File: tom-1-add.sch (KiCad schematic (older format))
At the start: 5 parts, among them J9 Conn_02x08_Top_Bottom, U12 74LS283, U13 74LS283, U18 74LS283, U19 74LS283

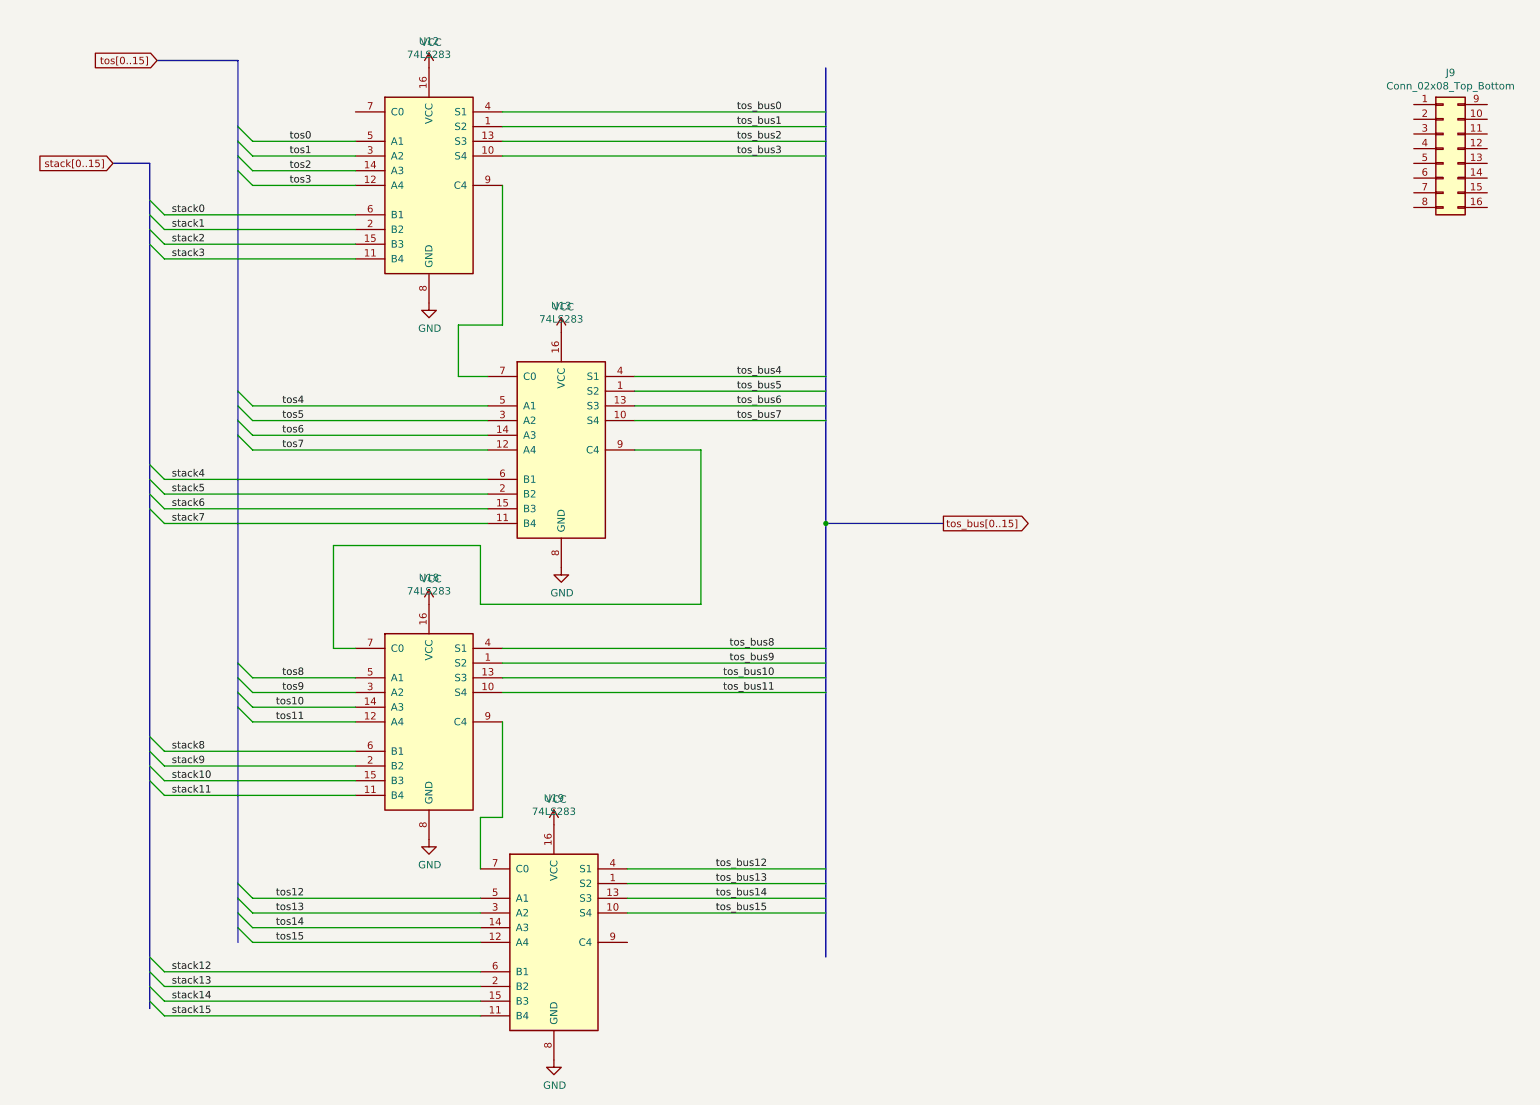
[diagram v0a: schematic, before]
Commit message: Next level
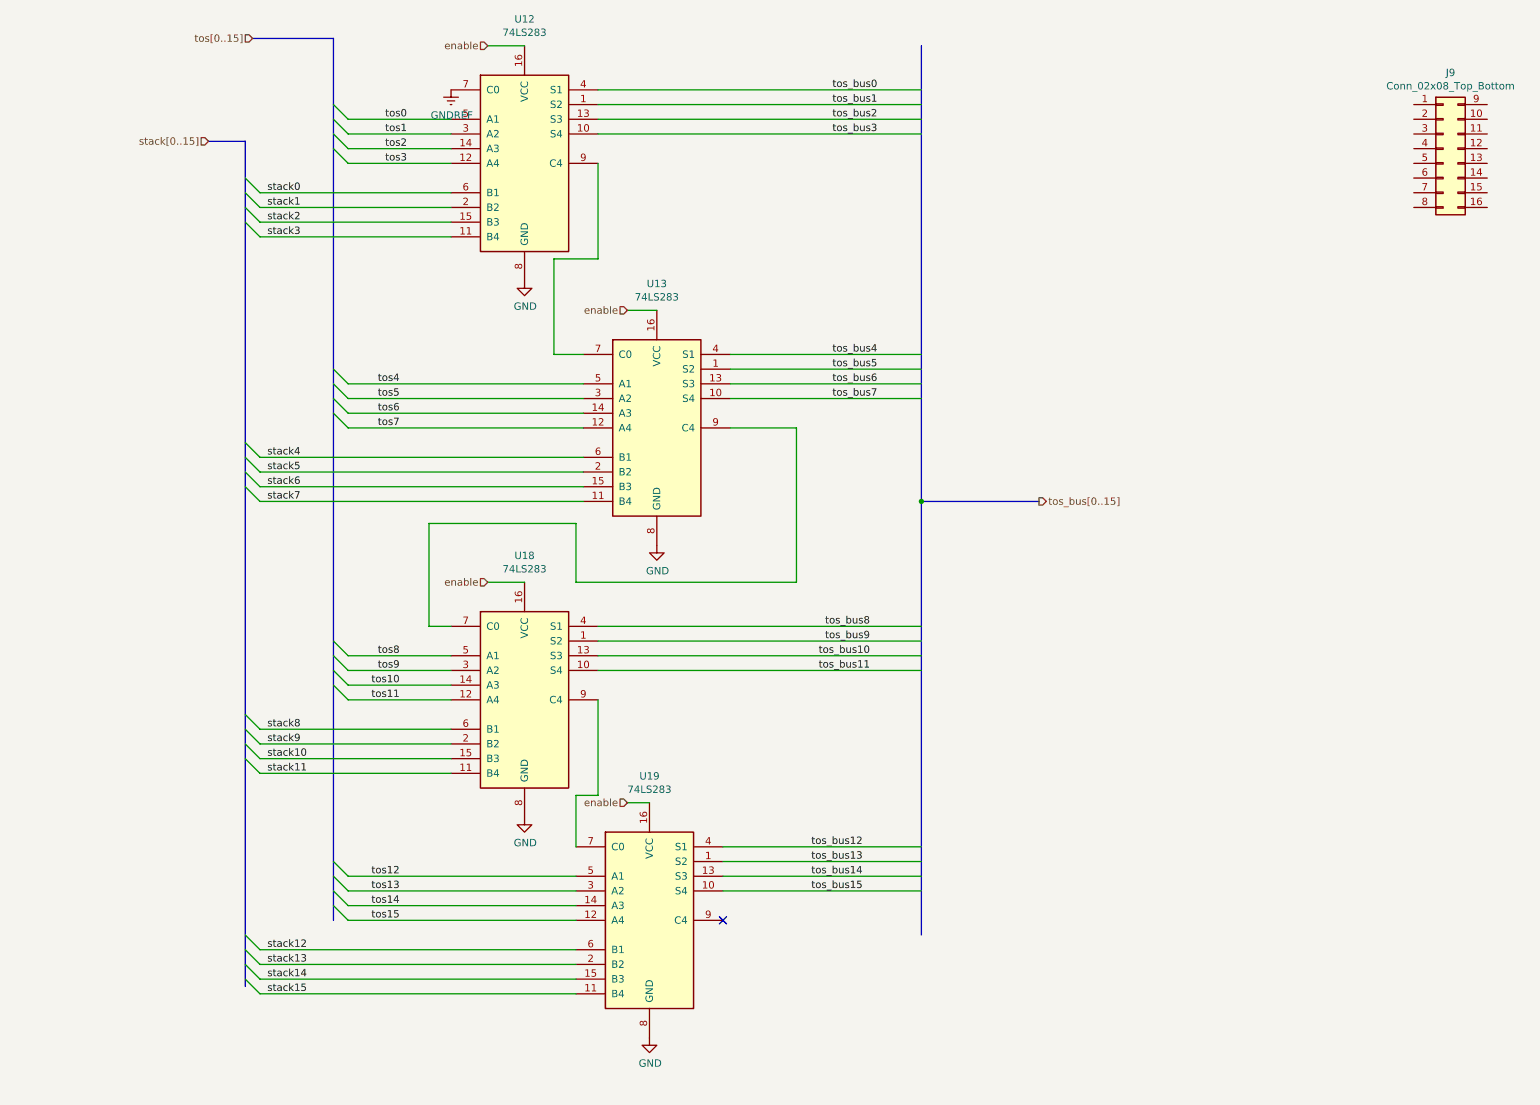
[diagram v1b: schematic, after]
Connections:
- net labels added: GNDREF, enable
- net labels removed: VCC
- wire segments 62 -> 66
- no-connect marks 0 -> 1
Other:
- moved on the sheet: U12, U13, U18, U19
